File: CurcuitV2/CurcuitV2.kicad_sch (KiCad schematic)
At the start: 83 parts, among them IC1 AS5600-ASOT, J1 Conn_01x07, J2 Conn_01x03, J3 Conn_01x02, J4 Conn_01x02, Q1 Q_NMOS_DGS, Q2 Q_NMOS_DGS, Q3 Q_NMOS_DGS, Q4 Q_NMOS_DGS, Q5 Q_NMOS_DGS, Q6 Q_NMOS_DGS, SW1 SW_Push, SW2 SW_Push, U1 DRV8300DPWR, U2 STM32F303K8Tx, U3 MCP9700x-ETT, U7 AP7375-3.3, Y2 CSTNE16M0V530000R0

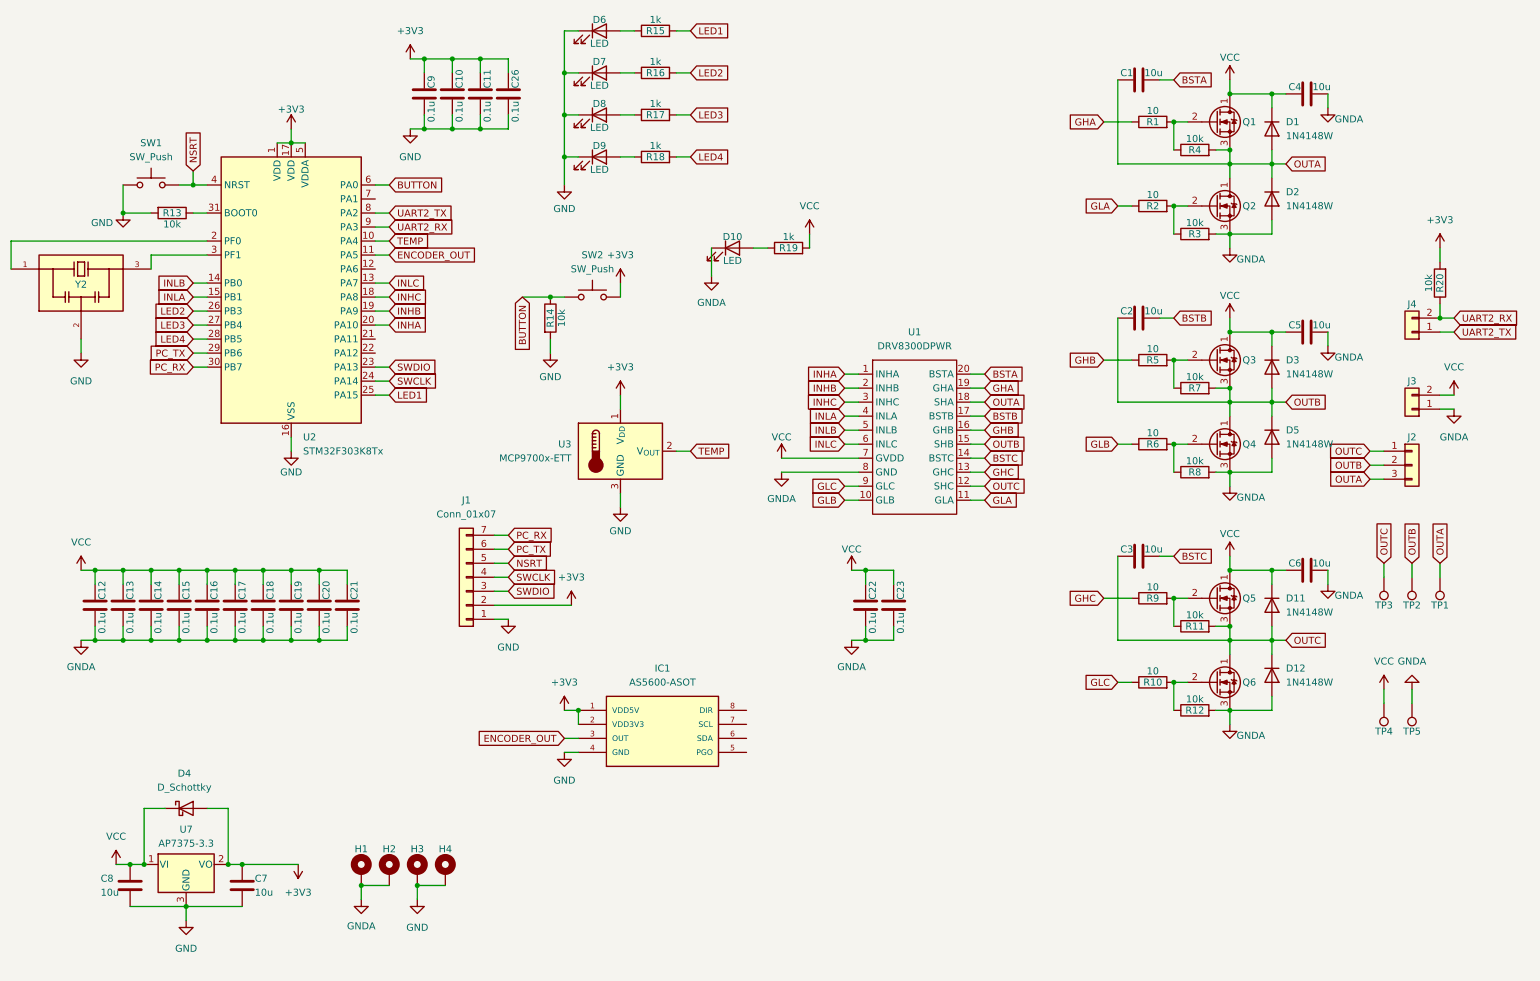
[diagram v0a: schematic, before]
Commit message: 完成
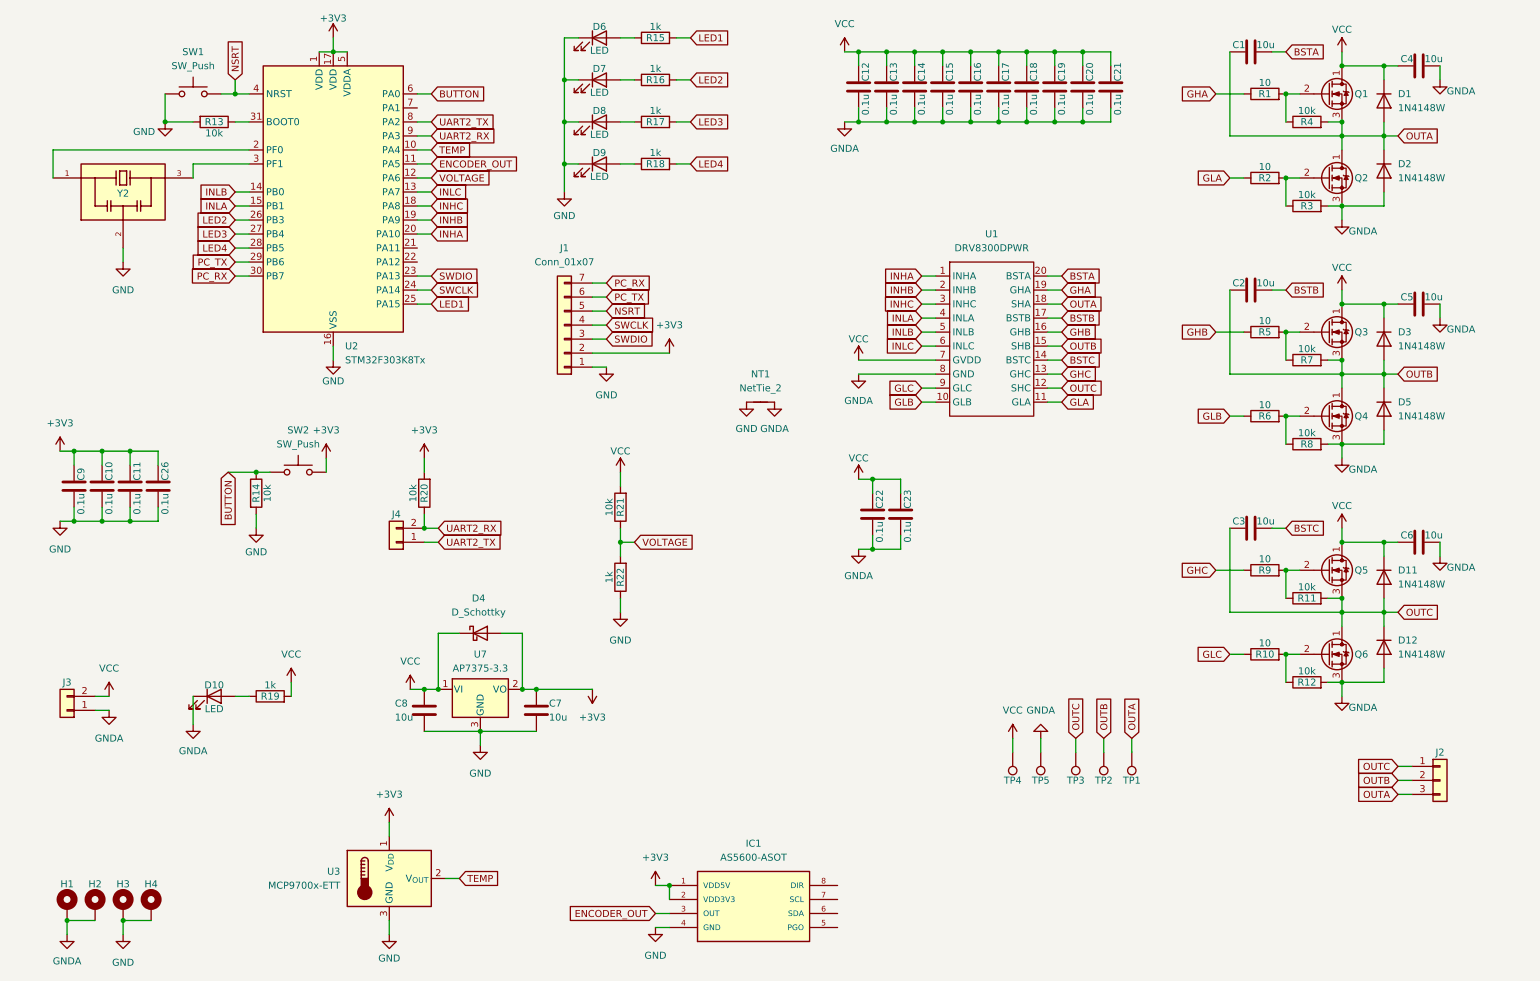
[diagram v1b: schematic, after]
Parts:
- added NT1: NetTie_2, NetTie:NetTie-2_SMD_Pad2.0mm, symbol Device:NetTie_2
- added R21: 10k, Resistor_SMD:R_0603_1608Metric, symbol Device:R
- added R22: 1k, Resistor_SMD:R_0603_1608Metric, symbol Device:R
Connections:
- net GND: now also NT1.1, R22.1
- net GNDA: now also NT1.2
- net VCC: now also R21.2
- net VOLTAGE: now reaches U2.12 (PA6)
- net VOLTAGE: now also R21.1, R22.2
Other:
- moved on the sheet: C1, C10, C11, C12, C13, C14, C15, C16, C17, C18, C19, C2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
